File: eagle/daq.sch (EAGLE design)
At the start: 77 parts

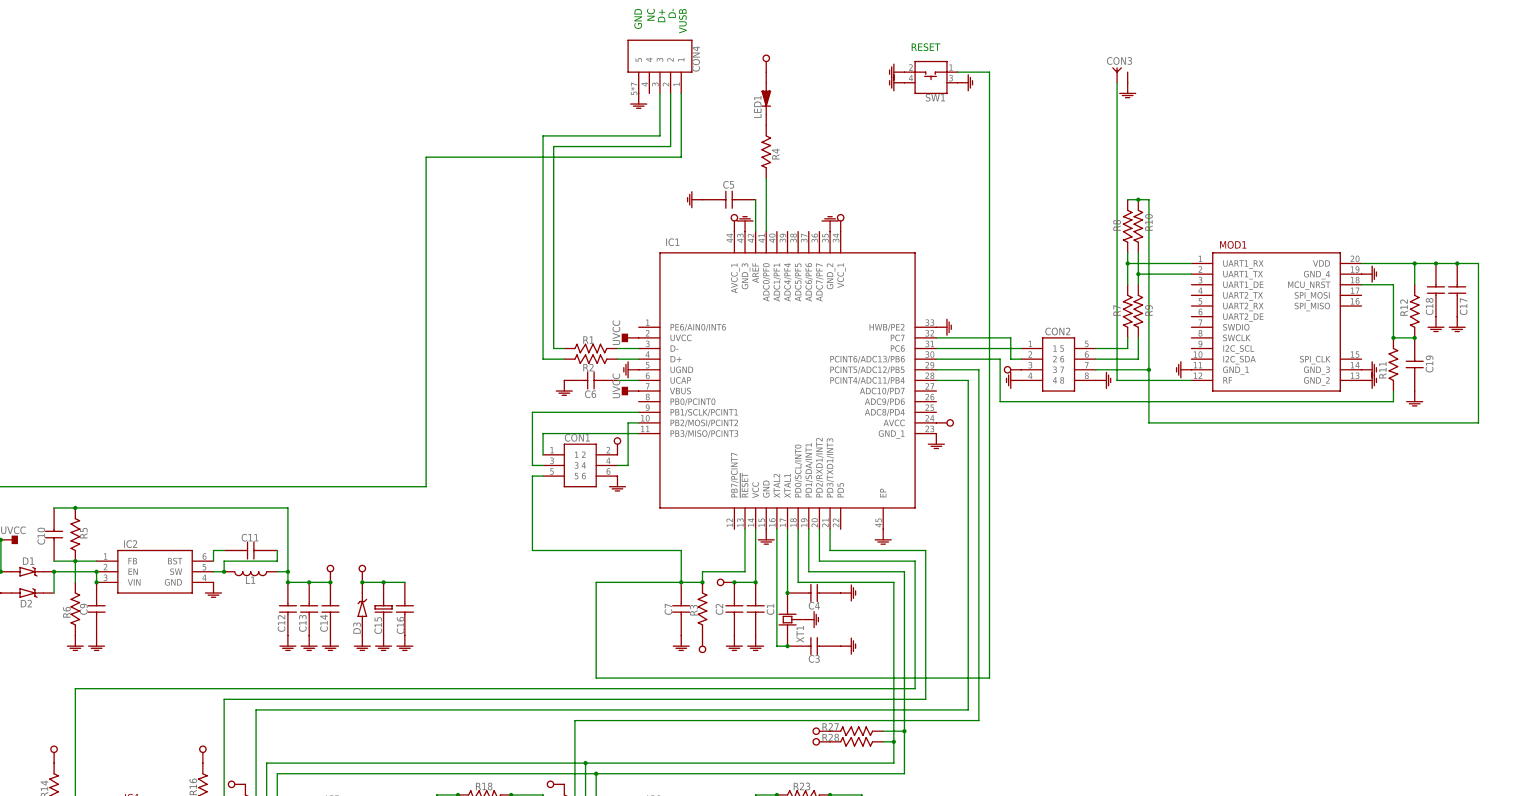
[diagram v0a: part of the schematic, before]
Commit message: do
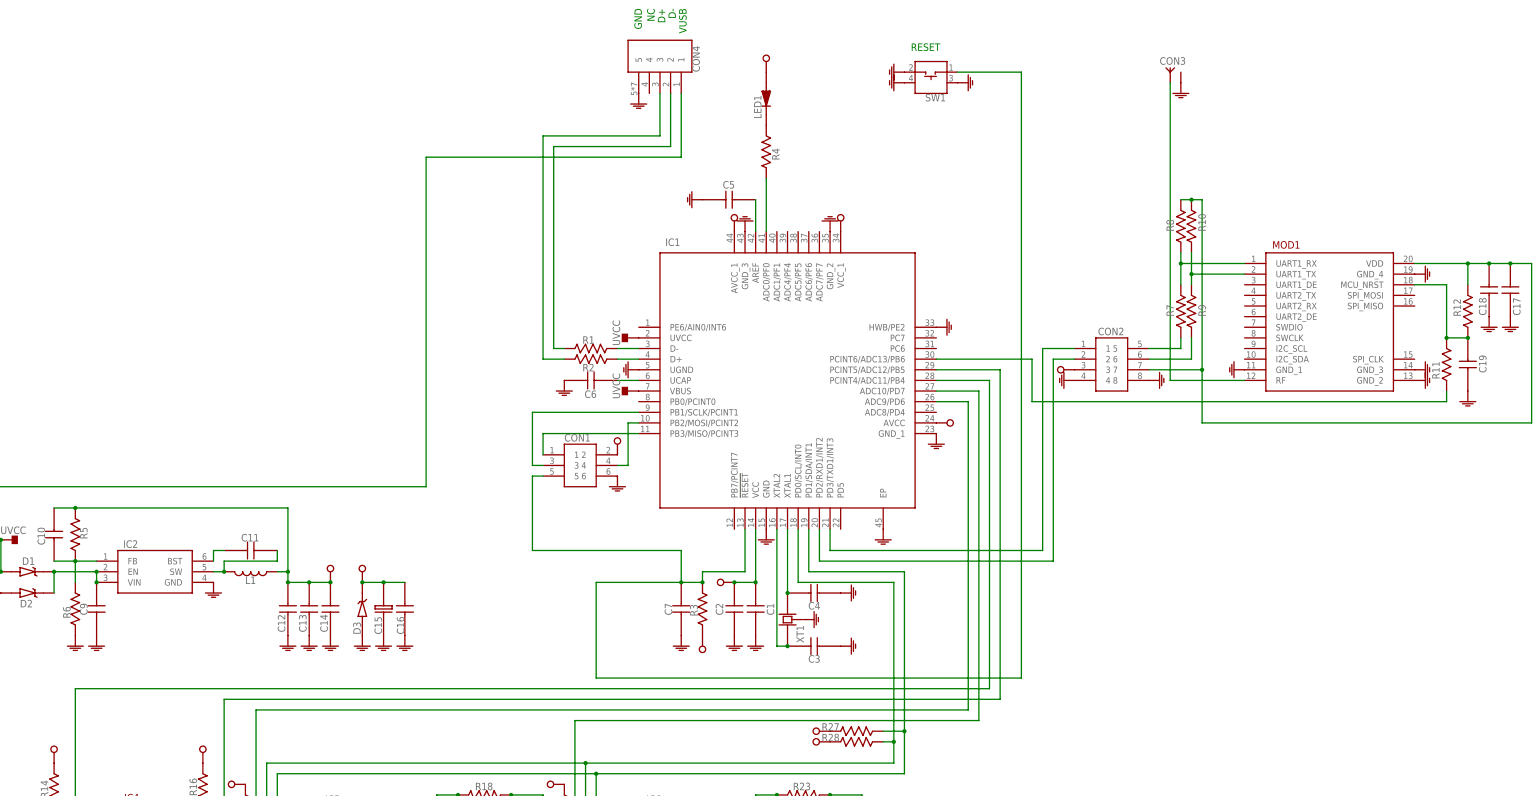
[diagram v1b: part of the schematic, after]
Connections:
- removed net N$11: CON2.1, IC1.PC6
- removed net N$5: CON2.2, IC1.PC7
- new net N$24: CON2.1, IC1.PD3/TXD1/INT3
- new net N$25: CON2.2, IC1.PD2/RXD1/INT2
- net N$15: now also IC1.ADC10/PD7; no longer IC1.PCINT5/ADC12/PB5
- net N$23: now also IC1.ADC9/PD6; no longer IC1.PCINT4/ADC11/PB4
- net N$32: now also IC1.PCINT5/ADC12/PB5; no longer IC1.PD3/TXD1/INT3
- net N$35: now also IC1.PCINT4/ADC11/PB4; no longer IC1.PD2/RXD1/INT2
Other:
- moved on the sheet: C17, C18, C19, CON2, CON3, MOD1, R10, R11, R12, R7, R8, R9
